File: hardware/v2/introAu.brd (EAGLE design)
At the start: 61.4 x 53.2 mm, 26 parts

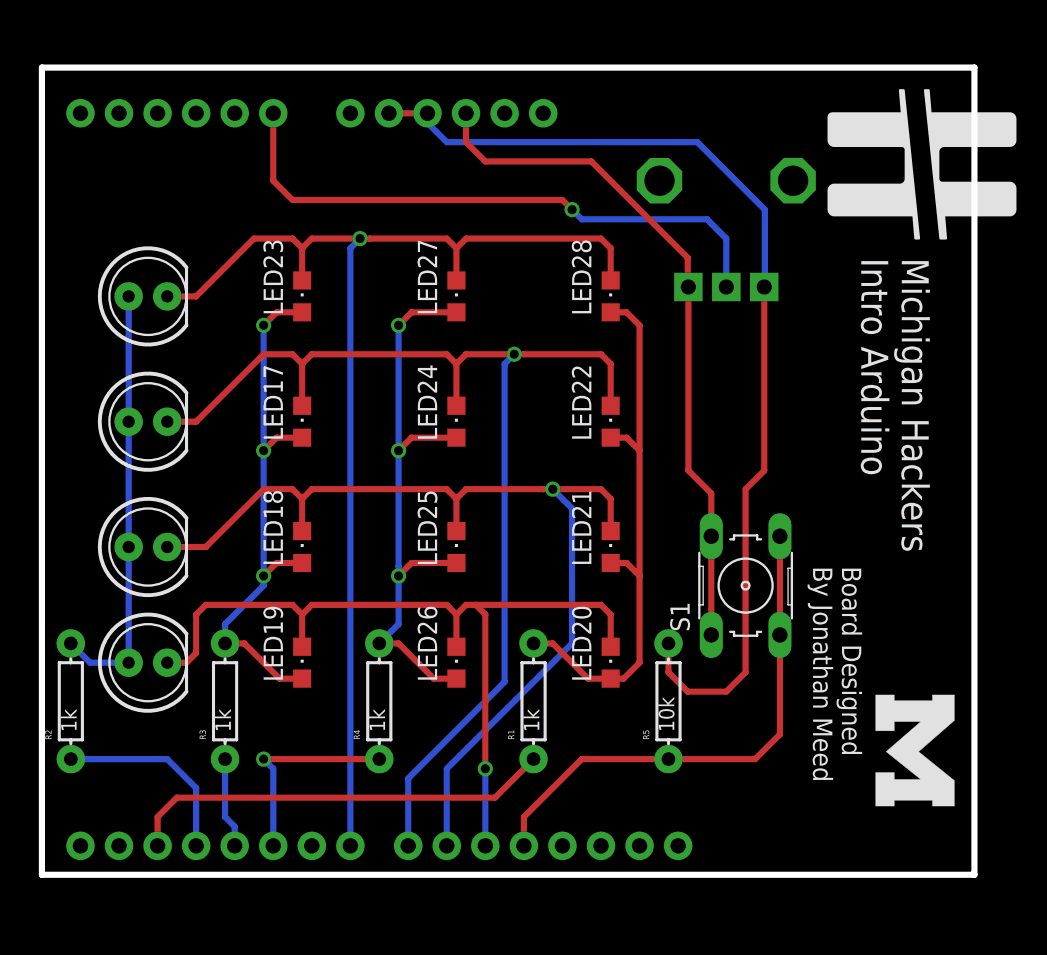
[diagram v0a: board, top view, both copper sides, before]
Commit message: Merged in Leonardo onboard
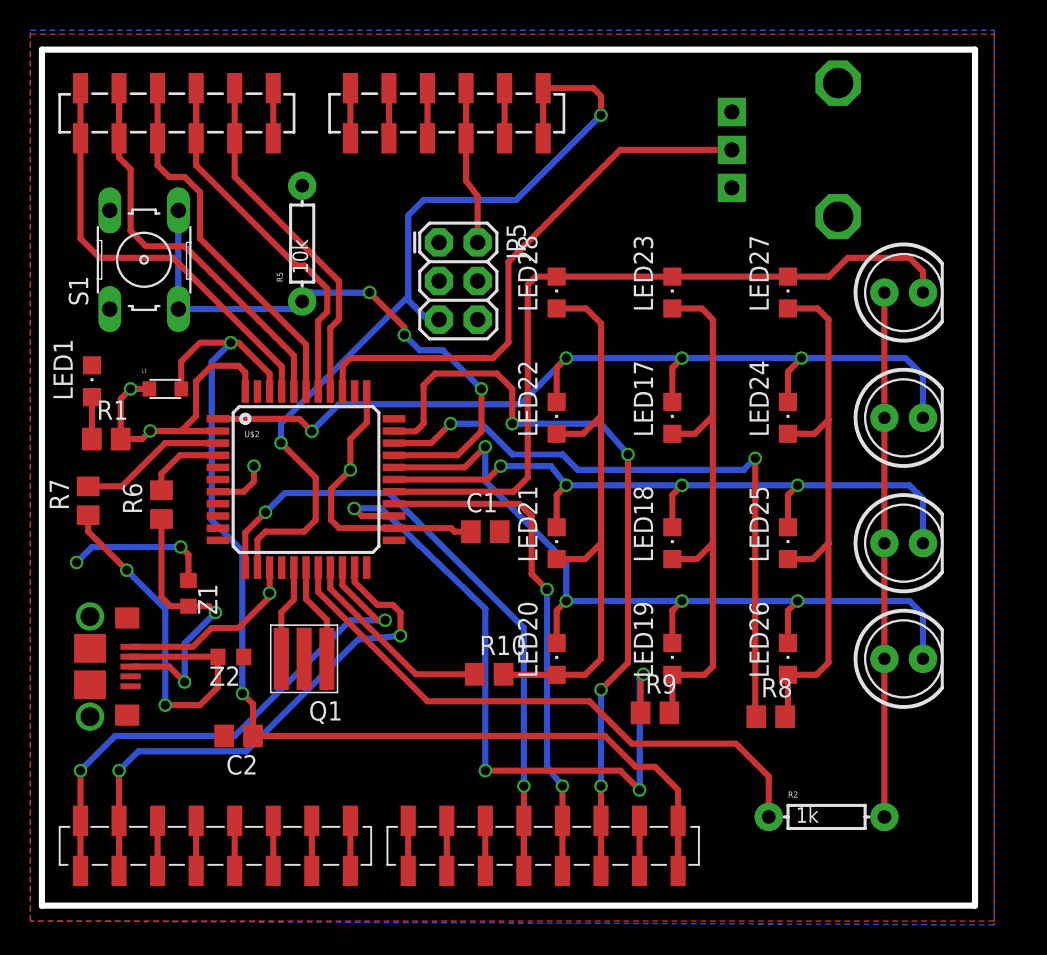
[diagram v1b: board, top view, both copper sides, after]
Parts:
- removed R3, R4: 1k, SparkFun-Resistors:AXIAL-0.3EZ
- removed U$1: ARDUINO_SHIELDNO_SILK, SparkFun-Boards:DUEMILANOVE_VIAS
- added C1, C2: 100nF, rcl:C0805
- added JP1, JP2: (no value), SparkFun-Connectors:1X06_SMD_STRAIGHT_COMBO
- added JP3, JP4: (no value), SparkFun-Connectors:1X08_SMD_COMBINED
- added JP5: (no value), SparkFun-Connectors:2X3
- added L1: (no value), EagleLibrary_Wuerth_Elektronik_eiSos_rev15c:WE-CBF_0805(W=3.0)
- added LED1: (no value), led:CHIPLED_0805
- added Q1: CERAMIC_RESONATOR_SMD6M00G53Z, MESH_Arduino:CERAMIC_RESONATOR_SMD
- added R10, R8, R9: 1k, rcl:R0805
- added R6, R7: 22, rcl:R0805
- added Z1: zenor 3.6w, rcl:R0603
- added Z2: zener 3.6w, rcl:R0603
- R1: device SparkFun-Resistors:AXIAL-0.3EZ -> rcl:R0805
- U$2: value (none) -> ATMEGA32U4TQFP; device artwork:SMALL-M -> SparkFun-DigitalIC:SPARKFUN-DIGITALIC_TQFP44
- U$3: value (none) -> USB_MICROB_0001LF; device artwork:SMALL-MH -> mBLE:USB_MICROB_CHEAPER
- moved U$3 58.9 mm to (5.84, 13.7)
- moved R2 50.4 mm to (51.7, 3.81), turned to 0 degrees
- moved LED10 49.8 mm to (56.8, 21.8)
- moved LED14 49.8 mm to (56.8, 14.2)
- moved LED4 49.8 mm to (56.8, 38.4)
- moved LED9 49.8 mm to (56.8, 30.1)
- moved S1 45.1 mm to (6.73, 40.5)
- moved U$2 40.1 mm to (17.4, 26.0), turned to 0 degrees
- moved R5 38.6 mm to (17.1, 41.6)
- moved R1 33.0 mm to (4.24, 28.7), turned to 0 degrees
- moved LED17 24.4 mm to (41.5, 30.1)
- moved LED18 24.4 mm to (41.5, 21.8)
- moved LED19 24.4 mm to (41.5, 14.2)
- moved LED23 24.4 mm to (41.5, 38.4)
- moved LED24 21.8 mm to (49.1, 30.1)
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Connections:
- removed net N$16: R1.P$1, U$1.D2
- removed net N$17: R2.P$1, U$1.D3
- removed net N$18: R3.P$1, U$1.D4
- removed net N$19: R4.P$1, U$1.D5
- new net +3V3: JP2.2
- new net A0: JP1.1
- new net A1: JP1.2, U$2.37
- new net A2: JP1.3, U$2.38
- new net A3: JP1.4, U$2.39
- new net A4: JP1.5, U$2.40
- new net A5: JP1.6, U$2.41
- new net AREF: C2.1, JP4.1, L1.2, U$2.42
- new net D0: JP3.8, U$2.20
- new net D1: JP3.7, U$2.21
- new net D10: JP4.6
- new net D11: JP4.5, U$2.12
- new net D12: JP4.4, U$2.26
- new net D13: JP4.3, U$2.32
- new net D14: U$2.11
- new net D15: U$2.9
- new net D16: U$2.10
- new net D17: U$2.8
- new net D2: JP3.6
- new net D3: JP3.5
- new net D4: JP3.4
- new net D5: JP3.3
- new net D6: JP3.2
- new net D7: JP3.1
- new net D8: JP4.8
- new net D9: JP4.7
- new net MISO: JP5.1
- new net MOSI: JP5.4
- new net N$1: R10.1, U$2.19
- new net N$11: LED1.A, R1.1
- new net N$2: R2.P$1, U$2.18
- new net N$3: R9.1, U$2.25
- new net N$4: R8.1, U$2.31
- new net N$5: Q1.3, U$2.16
- new net N$6: Q1.1, U$2.17
- new net N$7: R7.1, U$3.P$2, Z2.2
- new net N$9: R6.1, U$3.P$3, Z1.2
- new net RD+: R6.2, U$2.4
- new net RD-: R7.2, U$2.3
- new net RESET: JP2.1, JP5.5, U$2.13
- new net SCK: JP5.3
- new net TX: U$2.22
- new net VIN: JP2.6
- net +5V: now also C1.1, JP2.3, JP5.2, L1.1, R1.2, U$2.14, U$2.2, U$2.24, U$2.34, U$2.44, U$2.7, U$3.P$1; no longer U$1.5V
- net BUTTON: now also U$2.30; no longer U$1.D11
- net COL1: now also U$2.27; no longer U$1.D7
- net COL2: now also U$2.1; no longer U$1.D8
- net COL3: now also U$2.28; no longer U$1.D9
- net COL4: now also U$2.29; no longer U$1.D10
- net GND: now also C1.2, C2.2, JP2.4, JP2.5, JP4.2, JP5.6, LED1.C, Q1.2, U$2.15, U$2.23, U$2.35, U$2.43, U$2.5, U$2.6, U$3.P$4, Z1.1, Z2.1; no longer U$1.GND@0, U$1.GND@1
- net POT: now also U$2.36; no longer U$1.A0
- net ROW1: now also R10.2; no longer R1.P$2
- net ROW3: now also R9.2; no longer R3.P$2
- net ROW4: now also R8.2; no longer R4.P$2
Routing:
- net AREF: track 0.00 -> 72.5 mm, vias 0 -> 2
- net GND: track 66.8 -> 9.69 mm, vias 0 -> 2
- net RESET: track 0.00 -> 54.2 mm, vias 0 -> 2
- net D13: track 0.00 -> 50.3 mm, vias 0 -> 4
- net N$3: track 0.00 -> 45.8 mm, vias 0 -> 4
- net N$4: track 0.00 -> 42.9 mm, vias 0 -> 2
- net D11: track 0.00 -> 41.4 mm, vias 0 -> 2
- net N$2: track 0.00 -> 39.0 mm
- net D1: track 0.00 -> 35.1 mm, vias 0 -> 2
- net D0: track 0.00 -> 32.4 mm, vias 0 -> 2
- net D12: track 0.00 -> 30.2 mm, vias 0 -> 2
- net COL1: track 78.7 -> 50.4 mm, vias 1 -> 0
- net N$16: track 28.2 -> 0.00 mm
- net N$7: track 0.00 -> 26.3 mm, vias 0 -> 2
- net A4: track 0.00 -> 26.2 mm
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- added copper zone on layer 16, net +5V
- added copper zone on layer 1, net GND
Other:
- board size 61.4 x 53.2 mm -> 61.5 x 56.4 mm
- board text removed: "Board Designed By Jonathan Meed"
- board text removed: "Michigan Hackers Intro Arduino"
